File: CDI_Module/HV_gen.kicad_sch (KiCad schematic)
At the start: 10 parts, among them Q2 IRF3205, U1 NE555P

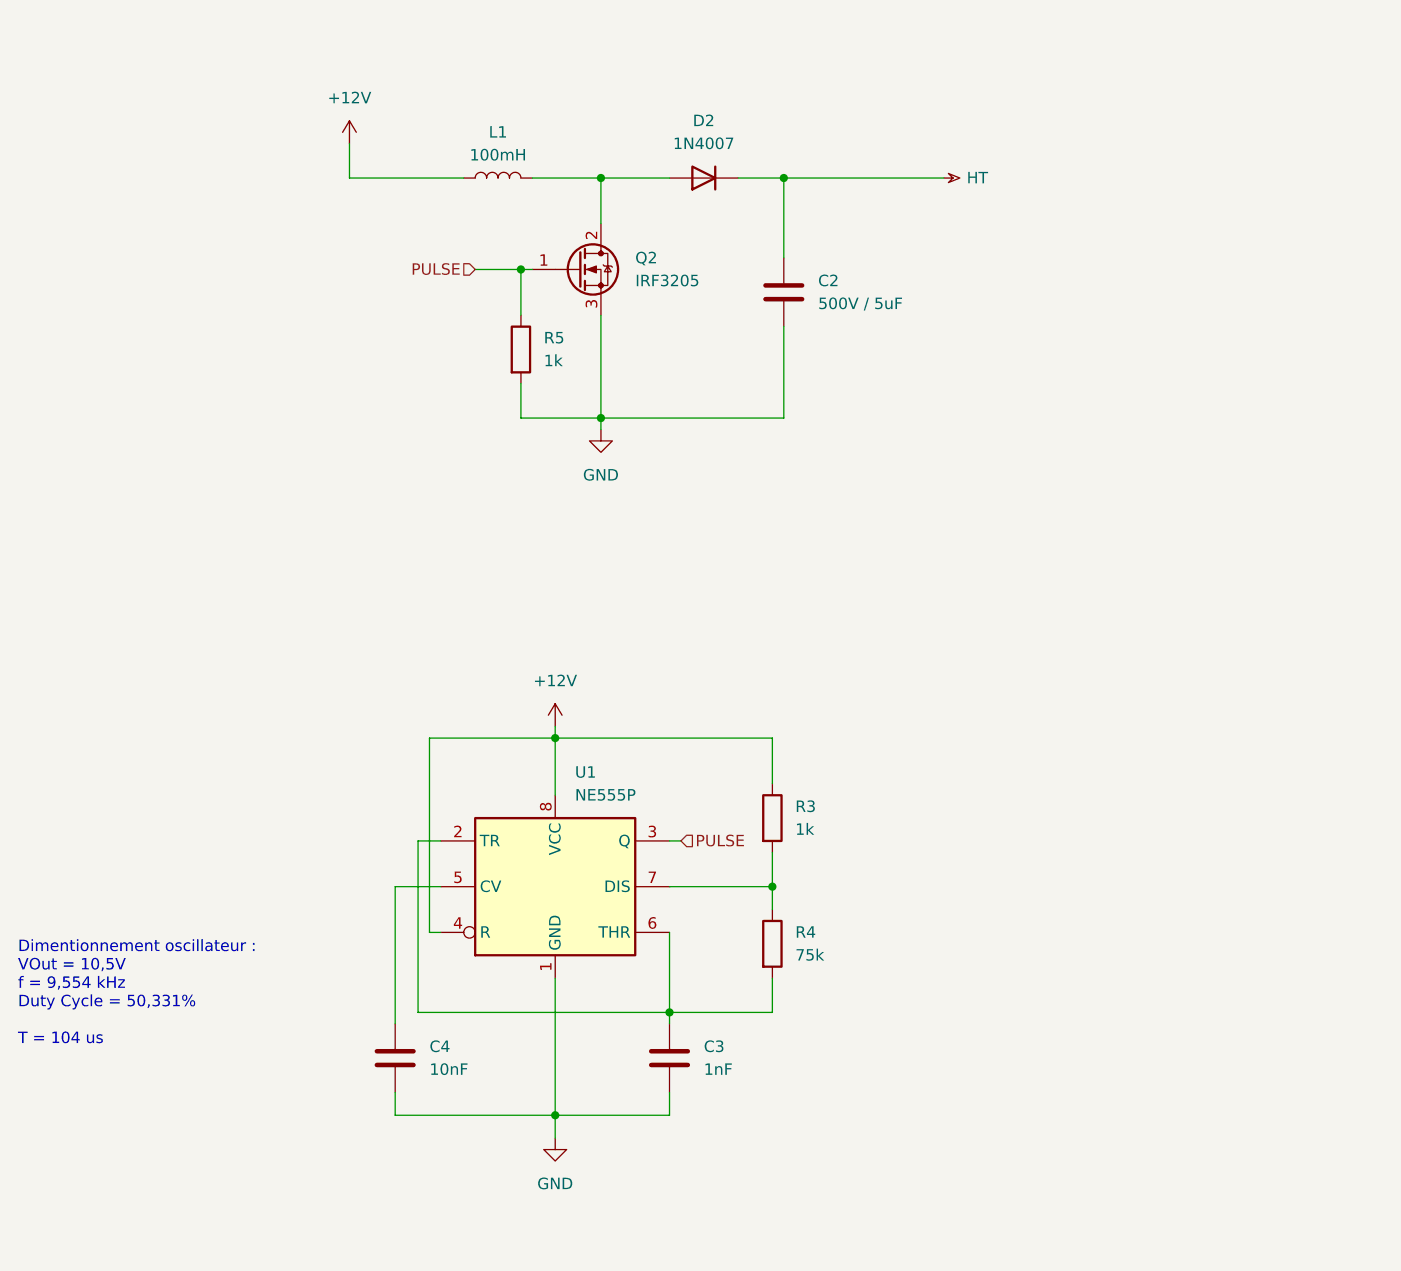
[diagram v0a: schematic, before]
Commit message: Test montage générateur de Haute tension
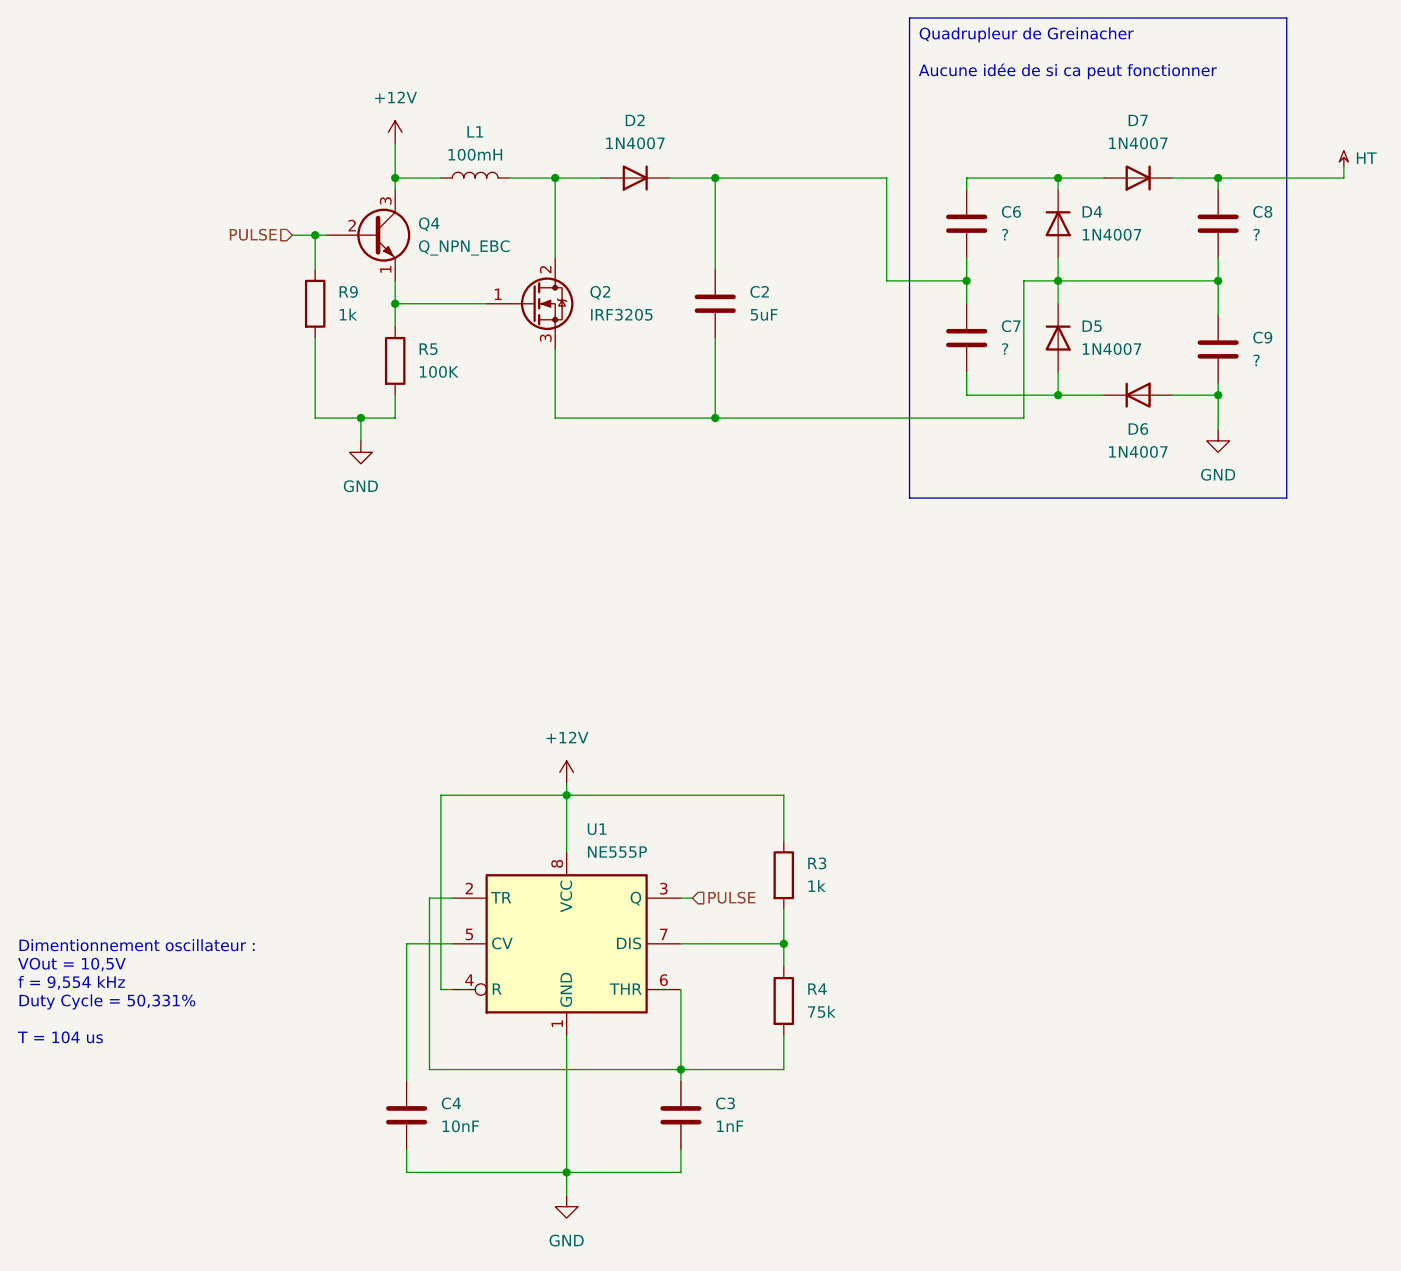
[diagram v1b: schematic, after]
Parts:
- added C6, C7, C8, C9: ?, symbol Device:C
- added D4, D5, D6, D7: 1N4007, Diode_THT:D_DO-41_SOD81_P10.16mm_Horizontal, symbol Diode:1N4007
- added Q4: Q_NPN_EBC, symbol Device:Q_NPN_EBC
- added R9: 1k, Resistor_THT:R_Axial_DIN0204_L3.6mm_D1.6mm_P5.08mm_Horizontal, symbol Device:R
- C2: value 500V / 5uF -> 5uF
- R5: value 1k -> 100K
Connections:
- net +12V: now also Q4.3 (C)
- net GND: now also C9.2, D6.2 (A), R9.2; no longer C2.2, Q2.3 (S)
- net HT: now also C8.1, D7.1 (K); no longer C2.1, D2.1 (K)
- net PULSE: now also Q4.2 (B), R9.1; no longer Q2.1 (G), R5.1
- new net: C2.2, C8.2, C9.1, D4.2 (A), D5.1 (K), Q2.3 (S)
- new net: C6.1, D4.1 (K), D7.2 (A)
- new net: Q2.1 (G), Q4.1 (E), R5.1
- new net: C2.1, C6.2, C7.1, D2.1 (K)
- new net: C7.2, D5.2 (A), D6.1 (K)
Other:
- moved on the sheet: C2, C3, C4, D2, L1, Q2, R3, R4, R5, U1
